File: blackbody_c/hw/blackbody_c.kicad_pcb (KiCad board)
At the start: 2 copper layers, 7.8 x 7.8 mm, 7 parts, among them IC101 TSL25911FN

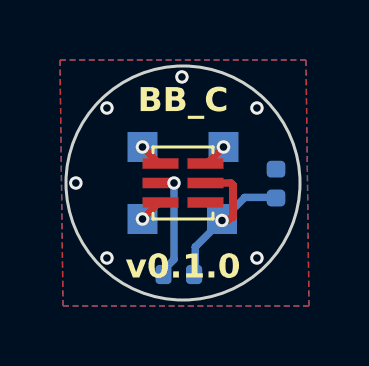
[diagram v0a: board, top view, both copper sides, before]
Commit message: blackbody c revisions based on review
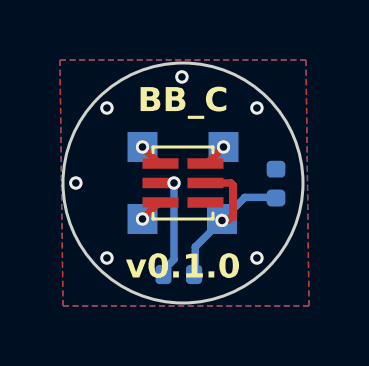
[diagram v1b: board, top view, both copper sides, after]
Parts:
- IC101: footprint footprints:TSL25911FN -> footprints:ams_TSL25911FN
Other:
- board size 7.8 x 7.8 mm -> 8 x 8 mm
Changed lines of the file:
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@@
   (net 5 "Net-(IC101-INT)")
   (net 6 "unconnected-(IC101-NC-Pad4)")
-  (footprint "footprints:TSL25911FN" (layer "F.Cu")
+  (footprint "footprints:ams_TSL25911FN" (layer "F.Cu")
     (at 100 50)
     (descr "TSL25911FN")
@@
     (attr smd)
     (fp_text reference "IC101" (at 0 0) (layer "F.SilkS") hide
-        (effects (font (size 0.8 0.8) (thickness 0.15)))
+        (effects (font (size 1.27 1.27) (thickness 0.254)))
     )
     (fp_text value "TSL25911FN" (at 0 0) (layer "F.SilkS") hide
-        (effects (font (size 0.8 0.8) (thickness 0.15)))
+        (effects (font (size 1.27 1.27) (thickness 0.254)))
     )
     (fp_text user "${REFERENCE}" (at 0 0) (layer "F.Fab")
-        (effects (font (size 0.8 0.8) (thickness 0.15)))
+        (effects (font (size 1.27 1.27) (thickness 0.254)))
     )
     (fp_line (start -1 -1.2) (end 1 -1.2)
@@
     (pad "6" smd rect (at 0.75 -0.65 90) (size 0.35 1.2) (layers "F.Cu" "F.Paste" "F.Mask")
       (net 4 "/SDA") (pinfunction "SDA") (pintype "passive"))
-    (model "${KIPRJMOD}/models/TSL25911FN.stp"
+    (model "${KIPRJMOD}/models/ams_TSL25911FN.stp"
       (offset (xyz 0 0 0.1))
       (scale (xyz 0.001 0.001 0.001))
@@
       (net 4 "/SDA") (pinfunction "1") (pintype "passive"))
   )
-  (gr_circle (center 100 50) (end 103.9 50)
+  (gr_circle (center 100 50) (end 104 50)
     (stroke (width 0.1) (type default)) (fill none) (layer "Edge.Cuts"))
-  (gr_text "-" (at 97.7 51.95) (layer "B.SilkS")
+  (gr_text "-" (at 98.6 53.1) (layer "B.SilkS")
     (effects (font (size 0.8 0.8) (thickness 0.15) bold) (justify left bottom mirror))
   )
-  (gr_text "SDA" (at 102.4 48) (layer "B.SilkS")
+  (gr_text "SDA" (at 102.4 47.9) (layer "B.SilkS")
     (effects (font (size 0.8 0.8) (thickness 0.15) bold) (justify left bottom mirror))
   )
-  (gr_text "SCL" (at 99.85 48) (layer "B.SilkS")
+  (gr_text "SCL" (at 99.6 47.9) (layer "B.SilkS")
     (effects (font (size 0.8 0.8) (thickness 0.15) bold) (justify left bottom mirror))
   )
-  (gr_text "+" (at 103.4 51.95) (layer "B.SilkS")
+  (gr_text "+" (at 102.2 53.2) (layer "B.SilkS")
     (effects (font (size 0.8 0.8) (thickness 0.15) bold) (justify left bottom mirror))
   )
@@
   )
   (dimension (type aligned) (layer "Dwgs.User")
-    (pts (xy 100 46.1) (xy 100 53.9))
+    (pts (xy 100 46) (xy 100 54))
     (height 5.5)
-    (gr_text "7.8000 mm" (at 93.55 50 90) (layer "Dwgs.User")
+    (gr_text "8.0000 mm" (at 93.55 50 90) (layer "Dwgs.User")
       (effects (font (size 0.8 0.8) (thickness 0.15)))
     )
